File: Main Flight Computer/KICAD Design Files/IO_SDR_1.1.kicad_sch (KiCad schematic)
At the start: 0 parts

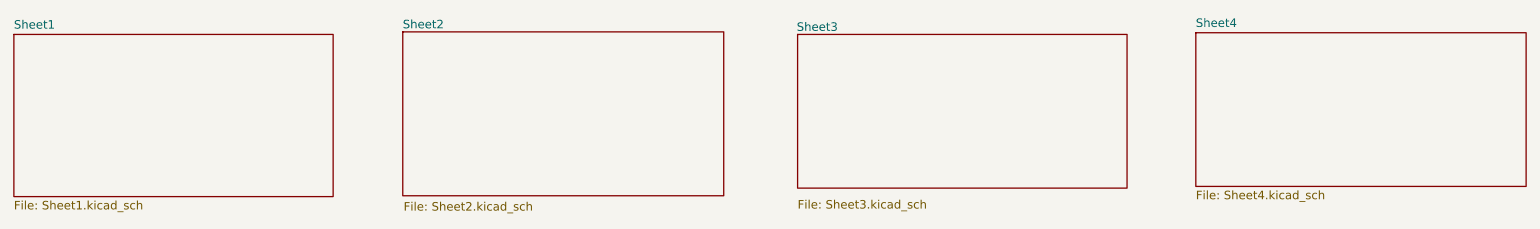
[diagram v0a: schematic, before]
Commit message: 1/14 Update
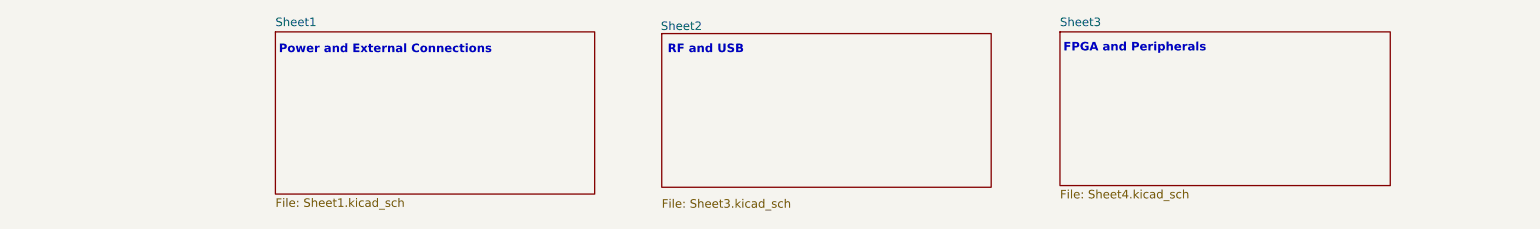
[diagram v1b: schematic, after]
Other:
- removed sheet Sheet4
- sheet Sheet2: file Sheet2.kicad_sch -> Sheet3.kicad_sch
- sheet Sheet3: file Sheet3.kicad_sch -> Sheet4.kicad_sch
- note added: "FPGA and Peripherals"
- note added: "Power and External Connections"
- note added: "RF and USB"
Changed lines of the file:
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@@
 	(generator_version "8.0")
 	(paper "A3")
+	(text "RF and USB"
+		(exclude_from_sim no)
+		(at 188.976 124.587 0)
+		(effects
+			(font
+				(size 1.27 1.27)
+				(thickness 0.508)
+				(bold yes)
+			)
+			(justify left bottom)
+		)
+	)
+	(text "Power and External Connections"
+		(exclude_from_sim no)
+		(at 130.81 124.587 0)
+		(effects
+			(font
+				(size 1.27 1.27)
+				(thickness 0.508)
+				(bold yes)
+			)
+			(justify left bottom)
+		)
+	)
+	(text "FPGA and Peripherals"
+		(exclude_from_sim no)
+		(at 248.158 124.333 0)
+		(effects
+			(font
+				(size 1.27 1.27)
+				(thickness 0.508)
+				(bold yes)
+			)
+			(justify left bottom)
+		)
+	)
 	(sheet
-		(at 208.407 121.539)
+		(at 188.087 121.412)
 		(size 49.276 22.987)
 		(stroke
@@
 			(color 0 0 0 0.0000)
 		)
-		(property "Sheetname" "Sheet3"
-			(at 208.28 121.158 0)
+		(property "Sheetname" "Sheet2"
+			(at 187.96 121.031 0)
 			(effects
 				(font
@@
 		)
 		(property "Sheetfile" "Sheet3.kicad_sch"
-			(at 208.407 146.2536 0)
+			(at 188.087 146.1266 0)
 			(effects
 				(font
@@
 	)
 	(sheet
-		(at 267.97 121.285)
+		(at 247.65 121.158)
 		(size 49.403 22.987)
 		(fields_autoplaced yes)
@@
 			(color 0 0 0 0.0000)
 		)
-		(property "Sheetname" "Sheet4"
-			(at 267.97 120.5734 0)
+		(property "Sheetname" "Sheet3"
+			(at 247.65 120.4464 0)
 			(effects
 				(font
@@
 		)
 		(property "Sheetfile" "Sheet4.kicad_sch"
-			(at 267.97 144.8566 0)
+			(at 247.65 144.7296 0)
 			(effects
 				(font
@@
 	)
 	(sheet
-		(at 149.352 121.158)
-		(size 48.006 24.511)
-		(stroke
-			(width 0.1524)
-			(type solid)
-		)
-		(fill
-			(color 0 0 0 0.0000)
-		)
-		(property "Sheetname" "Sheet2"
-			(at 149.352 120.777 0)
-			(effects
-				(font
-					(size 1.27 1.27)
-				)
-				(justify left bottom)
-			)
-		)
-		(property "Sheetfile" "Sheet2.kicad_sch"
-			(at 149.479 146.558 0)
-			(effects
-				(font
-					(size 1.27 1.27)
-				)
-				(justify left top)
-			)
-		)
-		(instances
-			(project "IO_SDR_1.1"
-				(path "/38786148-0fd1-46d3-8412-9a7876291ebf"
-					(page "2")
-				)
-			)
-		)
-	)
-	(sheet
-		(at 91.186 121.539)
+		(at 130.302 121.158)
 		(size 47.752 24.257)
 		(fields_autoplaced yes)
@@
 		)
 		(property "Sheetname" "Sheet1"
-			(at 91.186 120.8274 0)
+			(at 130.302 120.4464 0)
 			(effects
 				(font
@@
 		)
 		(property "Sheetfile" "Sheet1.kicad_sch"
-			(at 91.186 146.3806 0)
+			(at 130.302 145.9996 0)
 			(effects
 				(font
